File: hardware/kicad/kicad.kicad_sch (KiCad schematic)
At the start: 142 parts, among them J1 Conn_01x05, J2 USB_C_Receptacle_USB2.0, J3 Conn_01x08, SW1 MX_SW_solder, SW10 MX_SW_solder, SW11 MX_SW_solder, SW12 MX_SW_solder, SW13 MX_SW_solder, SW14 MX_SW_solder, SW15 MX_SW_solder, SW16 MX_SW_solder, SW17 MX_SW_solder, SW18 MX_SW_solder, SW19 MX_SW_solder, SW2 MX_SW_solder, SW20 MX_SW_solder, SW21 MX_SW_solder, SW22 MX_SW_solder, SW23 MX_SW_solder, SW24 MX_SW_solder, SW25 MX_SW_solder, SW26 MX_SW_solder, SW27 MX_SW_solder, SW28 MX_SW_solder, SW29 MX_SW_solder, SW3 MX_SW_solder, SW30 MX_SW_solder, SW31 MX_SW_solder, SW32 MX_SW_solder, SW33 MX_SW_solder, SW34 MX_SW_solder, SW35 MX_SW_solder, SW4 MX_SW_solder, SW5 MX_SW_solder, SW6 MX_SW_solder, SW7 MX_SW_solder, SW8 MX_SW_solder, SW9 MX_SW_solder, U1 RP2040, U2 W25Q128JVS, U3 XC6206PxxxMR, U4 USBLC6-2SC6, U5 74HC595, Y1 Crystal_GND24_Small

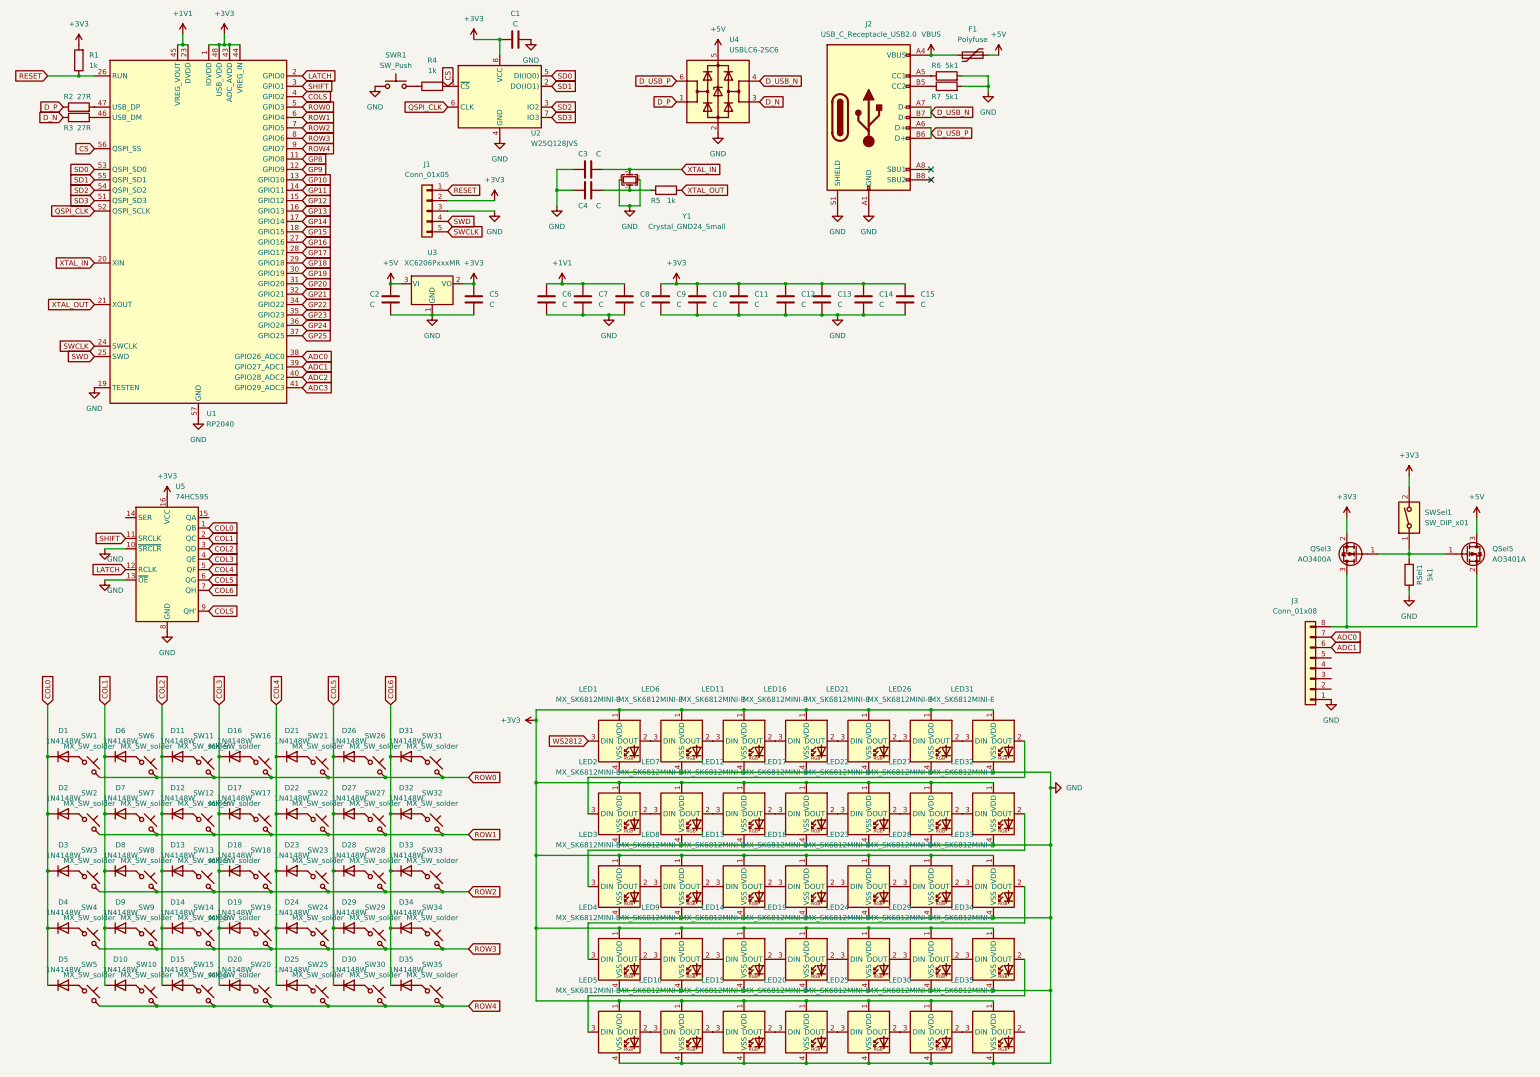
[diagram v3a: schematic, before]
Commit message: Update PCB
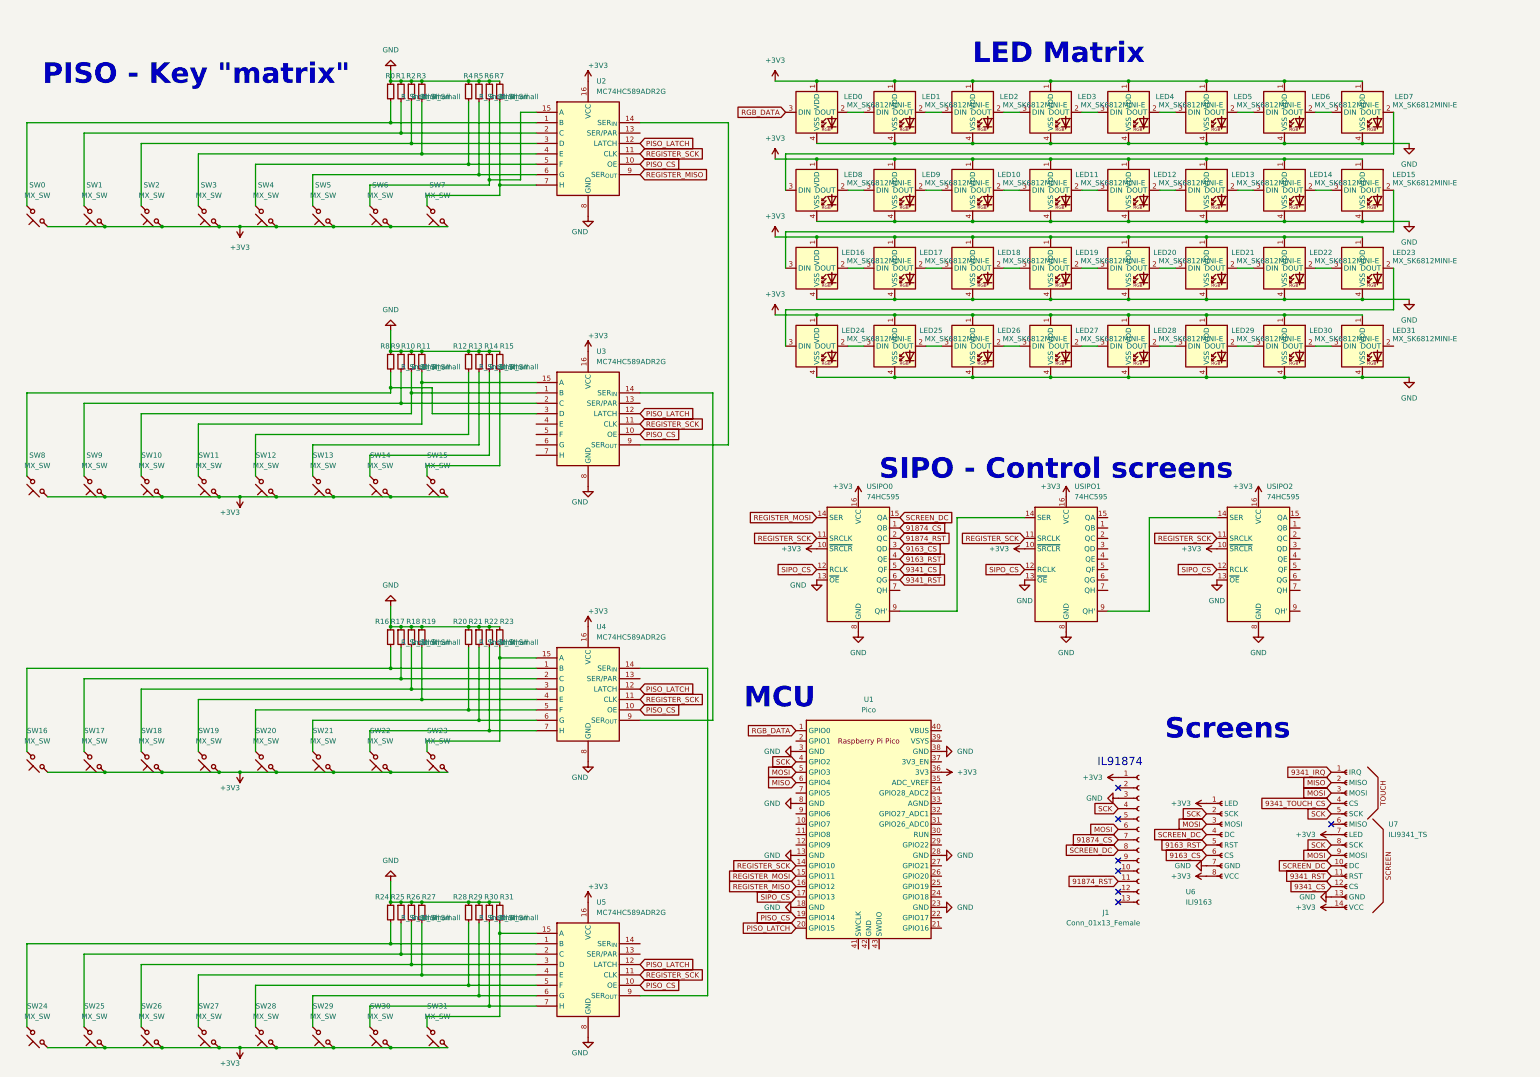
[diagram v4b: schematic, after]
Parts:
- removed C1, C10, C11, C12, C13, C14, C15, C2, C3, C4, C5, C6, C7, C8, C9: C, Capacitor_SMD:C_0603_1608Metric_Pad1.08x0.95mm_HandSolder, symbol Device:C
- removed D1, D10, D11, D12, D13, D14, D15, D16, D17, D18, D19, D2, D20, D21, D22, D23, D24, D25, D26, D27, D28, D29, D3, D30, D31, D32, D33, D34, D35, D4, D5, D6, D7, D8, D9: 1N4148W, Diode_SMD:D_SOD-123, symbol Diode:1N4148W
- removed F1: Polyfuse, Fuse:Fuse_0603_1608Metric_Pad1.05x0.95mm_HandSolder, symbol Device:Polyfuse
- removed J1: Conn_01x05, Connector_PinHeader_2.54mm:PinHeader_1x05_P2.54mm_Vertical, symbol Connector_Generic:Conn_01x05
- removed J2: USB_C_Receptacle_USB2.0, Connector_USB:USB_C_Receptacle_HRO_TYPE-C-31-M-12, symbol Connector:USB_C_Receptacle_USB2.0
- removed J3: Conn_01x08, Connector_PinHeader_2.54mm:PinHeader_1x08_P2.54mm_Vertical_SMD_Pin1Right, symbol Connector_Generic:Conn_01x08
- removed LED32, LED33, LED34, LED35: MX_SK6812MINI-E, marbastlib-mx:LED_MX_6028R, symbol marbastlib-mx:MX_SK6812MINI-E
- removed QSel3: AO3400A, Package_TO_SOT_SMD:SOT-23, symbol Transistor_FET:AO3400A
- removed QSel5: AO3401A, Package_TO_SOT_SMD:SOT-23, symbol Transistor_FET:AO3401A
- removed R1, R4, R5: 1k, Resistor_SMD:R_0603_1608Metric_Pad0.98x0.95mm_HandSolder, symbol Device:R
- removed R2, R3: 27R, Resistor_SMD:R_0603_1608Metric_Pad0.98x0.95mm_HandSolder, symbol Device:R
- removed R6, R7, RSel1: 5k1, Resistor_SMD:R_0603_1608Metric_Pad0.98x0.95mm_HandSolder, symbol Device:R
- removed SW1, SW10, SW11, SW12, SW13, SW14, SW15, SW16, SW17, SW18, SW19, SW2, SW20, SW21, SW22, SW23, SW24, SW25, SW26, SW27, SW28, SW29, SW3, SW30, SW31, SW32, SW33, SW34, SW35, SW4, SW5, SW6, SW7, SW8, SW9: MX_SW_solder, marbastlib-mx:SW_MX_1u, symbol marbastlib-mx:MX_SW_solder
- removed SWR1: SW_Push, Button_Switch_SMD:SW_SPST_TL3342, symbol Switch:SW_Push
- removed SWSel1: SW_DIP_x01, Button_Switch_SMD:SW_DIP_SPSTx01_Slide_6.7x4.1mm_W6.73mm_P2.54mm_LowProfile_JPin, symbol Switch:SW_DIP_x01
- removed U1: RP2040, Package_DFN_QFN:QFN-56-1EP_7x7mm_P0.4mm_EP3.2x3.2mm, symbol MCU_RaspberryPi:RP2040
- removed U2: W25Q128JVS, Package_SO:SOIC-8_5.23x5.23mm_P1.27mm, symbol Memory_Flash:W25Q128JVS
- removed U3: XC6206PxxxMR, Package_TO_SOT_SMD:SOT-23, symbol Regulator_Linear:XC6206PxxxMR
- removed U4: USBLC6-2SC6, Package_TO_SOT_SMD:SOT-23-6, symbol Power_Protection:USBLC6-2SC6
- removed U5: 74HC595, soic:SOIC16, symbol 74xx:74HC595
- removed Y1: Crystal_GND24_Small, Crystal:Crystal_SMD_3225-4Pin_3.2x2.5mm_HandSoldering, symbol Device:Crystal_GND24_Small
- added J1: Conn_01x13_Female, Connector_PinHeader_1.00mm:PinHeader_1x13_P1.00mm_Vertical, symbol Connector:Conn_01x13_Female
- added LED0: MX_SK6812MINI-E, marbastlib-mx:LED_MX_6028R, symbol marbastlib-mx:MX_SK6812MINI-E
- added R0, R1, R10, R11, R12, R13, R14, R15, R16, R17, R18, R19, R2, R20, R21, R22, R23, R24, R25, R26, R27, R28, R29, R3, R30, R31, R4, R5, R6, R7, R8, R9: R_Small, Resistor_SMD:R_1206_3216Metric_Pad1.30x1.75mm_HandSolder, symbol Device:R_Small
- added SW0, SW1, SW10, SW11, SW12, SW13, SW14, SW15, SW16, SW17, SW18, SW19, SW2, SW20, SW21, SW22, SW23, SW24, SW25, SW26, SW27, SW28, SW29, SW3, SW30, SW31, SW4, SW5, SW6, SW7, SW8, SW9: MX_SW, marbastlib-mx:SW_MX_1u, symbol marbastlib-mx:MX_SW_HS
- added U1: Pico, MCU_RaspberryPi_and_Boards:RPi_Pico_SMD_TH, symbol MCU_RaspberryPi_and_Boards:Pico
- added U2, U3, U4, U5: MC74HC589ADR2G, Package_SO:SO-16_3.9x9.9mm_P1.27mm, symbol my_components:MC74HC589ADR2G
- added U6: ILI9163, my_components:ILI9163, symbol my_components:ILI9163
- added U7: ILI9341_TS, my_components:ILI9341_TS, symbol my_components:ILI9341_TS
- added USIPO0, USIPO1, USIPO2: 74HC595, Package_SO:SO-16_3.9x9.9mm_P1.27mm, symbol 74xx:74HC595
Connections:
- net +3V3: now also J1.1 (Pin_1), LED0.1 (VDD), SW0.1, SW1.1, SW10.1, SW11.1, SW12.1, SW13.1, SW14.1, SW15.1, SW16.1, SW17.1, SW18.1, SW19.1, SW2.1, SW20.1, SW21.1, SW22.1, SW23.1, SW24.1, SW25.1, SW26.1, SW27.1, SW28.1, SW29.1, SW3.1, SW30.1, SW31.1, SW4.1, SW5.1, SW6.1, SW7.1, SW8.1, SW9.1, U1.36 (3V3), U2.16 (VCC), U3.16 (VCC), U4.16 (VCC), U5.16 (VCC), U6.1 (LED), U6.8 (VCC), U7.14 (VCC), U7.7 (LED), USIPO0.10 (~{SRCLR}), USIPO0.16 (VCC), USIPO1.10 (~{SRCLR}), USIPO1.16 (VCC), USIPO2.10 (~{SRCLR}), USIPO2.16 (VCC)
- net GND: now also J1.3 (Pin_3), LED0.4 (VSS), R0.1, R1.1, R10.1, R11.1, R12.1, R13.1, R14.1, R15.1, R16.1, R17.1, R18.1, R19.1, R2.1, R20.1, R21.1, R22.1, R23.1, R24.1, R25.1, R26.1, R27.1, R28.1, R29.1, R3.1, R30.1, R31.1, R4.1, R5.1, R6.1, R7.1, R8.1, R9.1, U1.13 (GND), U1.18 (GND), U1.23 (GND), U1.28 (GND), U1.3 (GND), U1.38 (GND), U1.8 (GND), U2.8 (GND), U3.8 (GND), U4.8 (GND), U5.8 (GND), U6.7 (GND), U7.13 (GND), USIPO0.13 (~{OE}), USIPO0.8 (GND), USIPO1.13 (~{OE}), USIPO1.8 (GND), USIPO2.13 (~{OE}), USIPO2.8 (GND)
- net at LED6.2 (DOUT): now also LED7.3 (DIN); no longer LED11.3 (DIN)
- net at LED1.2 (DOUT): now also LED2.3 (DIN); no longer LED6.3 (DIN)
- net at LED2.2 (DOUT): now also LED3.3 (DIN); no longer LED7.3 (DIN)
- net at LED31.2 (DOUT): no longer LED2.3 (DIN)
- net at LED22.3 (DIN): now also LED21.2 (DOUT); no longer LED17.2 (DOUT)
- net at LED12.2 (DOUT): now also LED13.3 (DIN); no longer LED17.3 (DIN)
- net at LED23.3 (DIN): now also LED22.2 (DOUT); no longer LED18.2 (DOUT)
- net at LED18.3 (DIN): now also LED17.2 (DOUT); no longer LED13.2 (DOUT)
- net at LED30.2 (DOUT): now also LED31.3 (DIN)
- net at LED28.3 (DIN): now also LED27.2 (DOUT); no longer LED23.2 (DOUT)
- net at LED29.2 (DOUT): now also LED30.3 (DIN)
- net at LED29.3 (DIN): now also LED28.2 (DOUT); no longer LED24.2 (DOUT)
- net at LED26.3 (DIN): now also LED25.2 (DOUT); no longer LED21.2 (DOUT)
- net at LED21.3 (DIN): now also LED20.2 (DOUT); no longer LED16.2 (DOUT)
- net at LED4.3 (DIN): now also LED3.2 (DOUT)
- net at LED26.2 (DOUT): now also LED27.3 (DIN); no longer LED31.3 (DIN)
- net at LED25.3 (DIN): now also LED24.2 (DOUT); no longer LED20.2 (DOUT)
- net at LED15.3 (DIN): now also LED14.2 (DOUT); no longer LED10.2 (DOUT)
- net at LED10.3 (DIN): now also LED9.2 (DOUT); no longer LED5.2 (DOUT)
- net at LED19.3 (DIN): now also LED18.2 (DOUT); no longer LED14.2 (DOUT)
- net at LED14.3 (DIN): now also LED13.2 (DOUT); no longer LED9.2 (DOUT)
- net at LED20.3 (DIN): now also LED19.2 (DOUT); no longer LED15.2 (DOUT)
- net at LED12.3 (DIN): now also LED11.2 (DOUT); no longer LED7.2 (DOUT)
- net at LED8.2 (DOUT): now also LED9.3 (DIN); no longer LED13.3 (DIN)
- net at LED8.3 (DIN): now also LED7.2 (DOUT); no longer LED3.2 (DOUT)
- net at LED24.3 (DIN): now also LED23.2 (DOUT); no longer LED19.2 (DOUT)
- net at LED4.2 (DOUT): now also LED5.3 (DIN); no longer LED9.3 (DIN)
- net at LED16.3 (DIN): now also LED15.2 (DOUT); no longer LED11.2 (DOUT)
- net WS2812: no longer names the net of LED1.3 (DIN)
- net WS2812: now also LED0.2 (DOUT)
- new net: R2.2, SW2.2, U2.3 (D)
- new net: R20.2, SW20.2, U4.5 (F)
- new net: R16.2, SW16.2, U4.1 (B)
- new net: R18.2, SW18.2, U4.3 (D)
- new net: R5.2, SW5.2, U2.6 (G)
- new net: R11.2, SW11.2, U3.15 (A)
- new net: R22.2, SW22.2, U4.7 (H)
- new net: R13.2, SW13.2
- new net: R9.2, SW9.2, U3.2 (C)
- new net: LED16.2 (DOUT), LED17.3 (DIN)
- new net: R31.2, SW31.2, U5.15 (A)
- new net: R6.2, SW6.2, U2.15 (A)
- new net: R3.2, SW3.2, U2.4 (E)
- new net: USIPO0.9 (QH'), USIPO1.14 (SER)
- new net: USIPO1.9 (QH'), USIPO2.14 (SER)
- new net: R14.2, SW14.2
- new net: R25.2, SW25.2, U5.2 (C)
- new net: R19.2, SW19.2, U4.4 (E)
- new net: R7.2, SW7.2, U2.7 (H)
- new net: R24.2, SW24.2, U5.1 (B)
- new net: R26.2, SW26.2, U5.3 (D)
- new net: R10.2, SW10.2, U3.1 (B)
- new net: U3.14 (SER_{IN}), U4.9 (SER_{OUT})
- new net: R8.2, SW8.2, U3.3 (D)
- new net: U2.14 (SER_{IN}), U3.9 (SER_{OUT})
- new net: U4.14 (SER_{IN}), U5.9 (SER_{OUT})
- new net: R23.2, SW23.2, U4.15 (A)
- new net: R17.2, SW17.2, U4.2 (C)
- new net: R21.2, SW21.2, U4.6 (G)
- new net: R4.2, SW4.2, U2.5 (F)
- new net: R1.2, SW1.2, U2.2 (C)
- new net: R30.2, SW30.2, U5.7 (H)
- new net: LED10.2 (DOUT), LED11.3 (DIN)
- new net: R12.2, SW12.2
- new net: R28.2, SW28.2, U5.5 (F)
- new net: R27.2, SW27.2, U5.4 (E)
- new net: R29.2, SW29.2, U5.6 (G)
- new net: R0.2, SW0.2, U2.1 (B)
- new net: R15.2, SW15.2
- new net: LED5.2 (DOUT), LED6.3 (DIN)
- new net 9163_CS: U6.6 (CS), USIPO0.3 (QD)
- new net 9163_RST: U6.5 (RST), USIPO0.4 (QE)
- new net 91874_CS: J1.7 (Pin_7), USIPO0.1 (QB)
- new net 91874_RST: J1.11 (Pin_11), USIPO0.2 (QC)
- new net 9341_CS: U7.12 (CS), USIPO0.5 (QF)
- new net 9341_IRQ: U7.1 (IRQ)
- new net 9341_RST: U7.11 (RST), USIPO0.6 (QG)
- new net 9341_TOUCH_CS: U7.4 (CS)
- new net MISO: U1.6 (GPIO4), U7.2 (MISO)
- new net MOSI: J1.6 (Pin_6), U1.5 (GPIO3), U6.3 (MOSI), U7.3 (MOSI), U7.9 (MOSI)
- new net PISO_CS: U1.19 (GPIO14), U2.10 (OE), U3.10 (OE), U4.10 (OE), U5.10 (OE)
- new net PISO_LATCH: U1.20 (GPIO15), U2.12 (LATCH), U3.12 (LATCH), U4.12 (LATCH), U5.12 (LATCH)
- new net REGISTER_MISO: U1.16 (GPIO12), U2.9 (SER_{OUT})
- new net REGISTER_MOSI: U1.15 (GPIO11), USIPO0.14 (SER)
- new net REGISTER_SCK: U1.14 (GPIO10), U2.11 (CLK), U3.11 (CLK), U4.11 (CLK), U5.11 (CLK), USIPO0.11 (SRCLK), USIPO1.11 (SRCLK), USIPO2.11 (SRCLK)
- new net RGB_DATA: LED0.3 (DIN), U1.1 (GPIO0)
- new net SCK: J1.4 (Pin_4), U1.4 (GPIO2), U6.2 (SCK), U7.5 (SCK), U7.8 (SCK)
- new net SCREEN_DC: J1.8 (Pin_8), U6.4 (DC), U7.10 (DC), USIPO0.15 (QA)
- new net SIPO_CS: U1.17 (GPIO13), USIPO0.12 (RCLK), USIPO1.12 (RCLK), USIPO2.12 (RCLK)
- no-connect marks 2 -> 7
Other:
- note added: "IL91874"
- note added: "LED Matrix"
- note added: "MCU"
- note added: "PISO - Key "matrix""
- note added: "SIPO - Control screens"
- note added: "Screens"
- title: (none) -> Access Keyboard

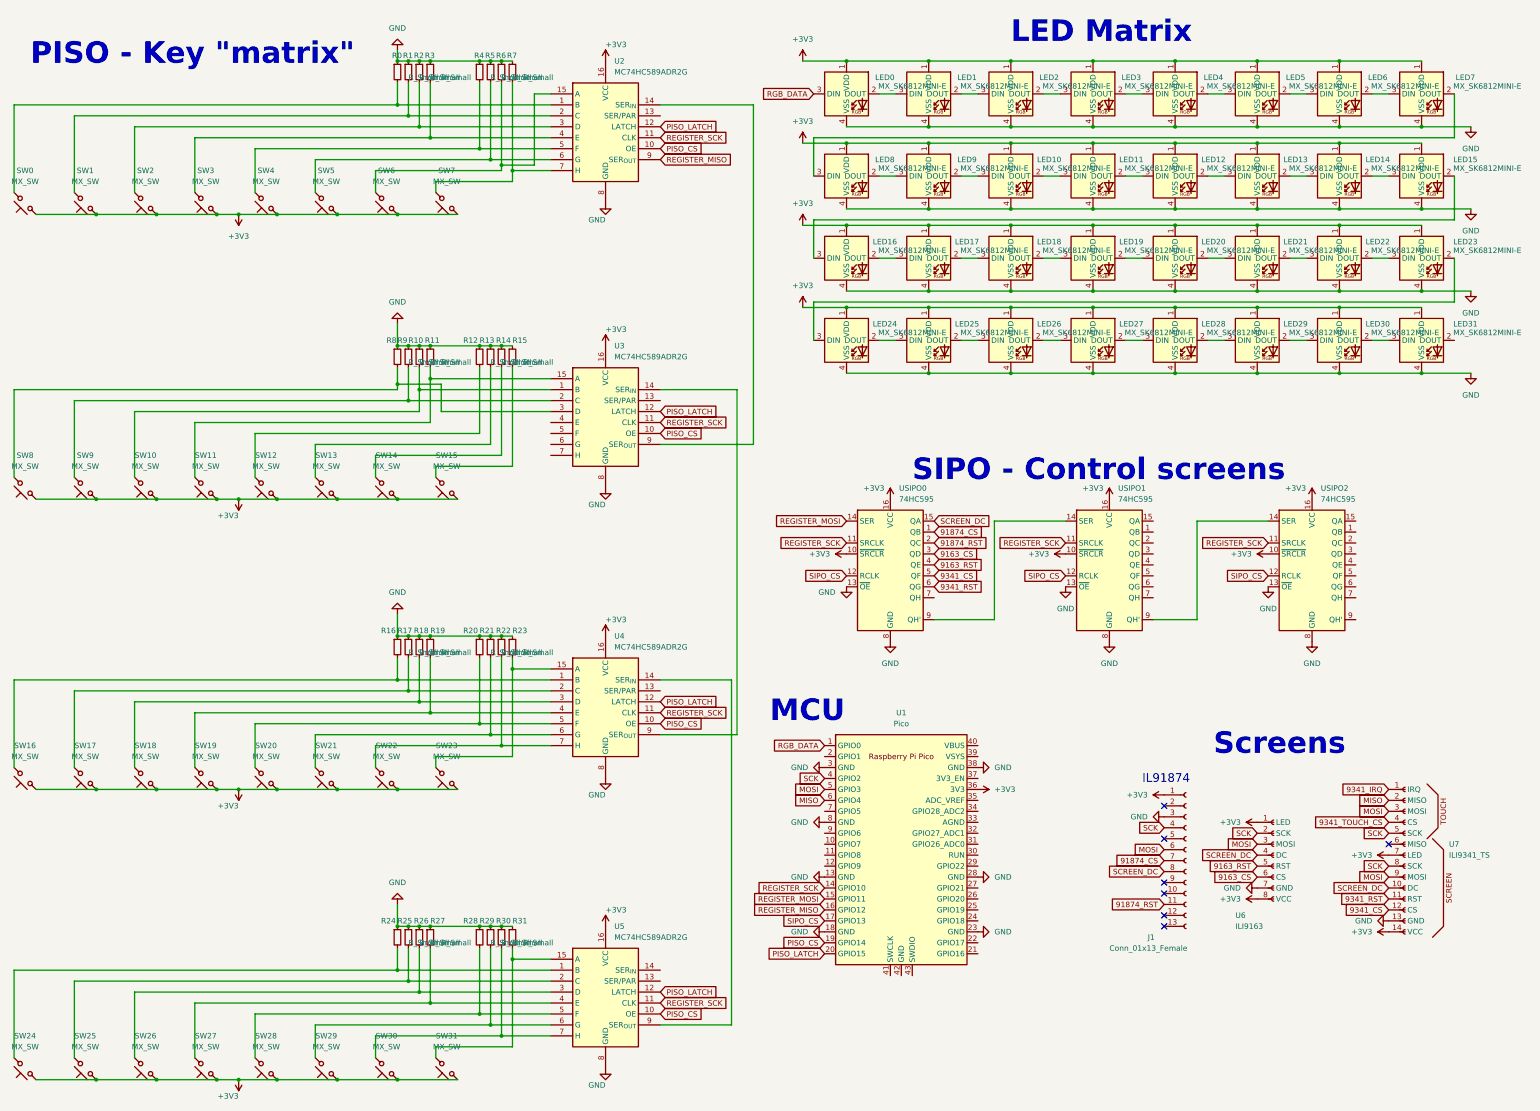
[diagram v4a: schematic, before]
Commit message: Matrix wired
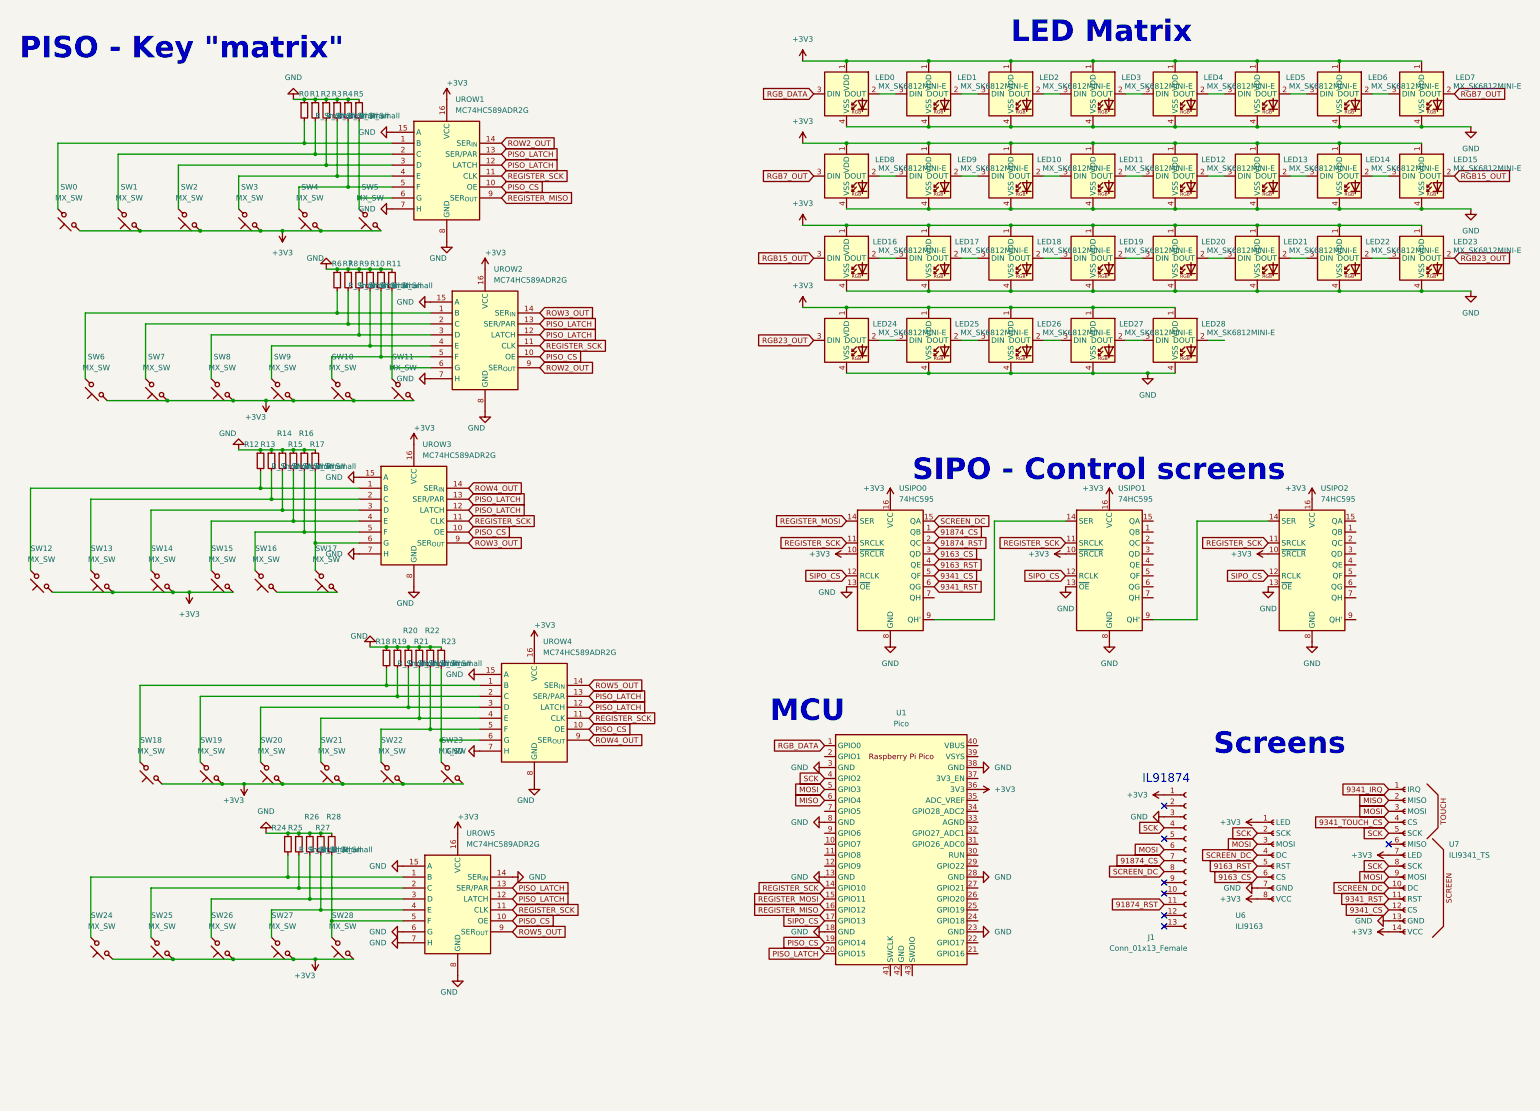
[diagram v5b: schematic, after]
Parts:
- removed LED29, LED30, LED31: MX_SK6812MINI-E, marbastlib-mx:LED_MX_6028R, symbol marbastlib-mx:MX_SK6812MINI-E
- removed R29, R30, R31: R_Small, Resistor_SMD:R_1206_3216Metric_Pad1.30x1.75mm_HandSolder, symbol Device:R_Small
- removed SW29, SW30, SW31: MX_SW, marbastlib-mx:SW_MX_1u, symbol marbastlib-mx:MX_SW_HS
- added UROW4: MC74HC589ADR2G, Package_SO:SO-16_3.9x9.9mm_P1.27mm, symbol my_components:MC74HC589ADR2G
- renumbered U2 to UROW1, U3 to UROW2, U4 to UROW3, U5 to UROW5
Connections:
- net +3V3: now also UROW4.16 (VCC); no longer SW16.1, SW17.1
- net GND: now also UROW1.15 (A), UROW1.7 (H), UROW2.15 (A), UROW2.7 (H), UROW3.15 (A), UROW3.7 (H), UROW5.14 (SER_{IN}), UROW5.15 (A), UROW5.6 (G), UROW5.7 (H), UROW4.15 (A), UROW4.7 (H), UROW4.8 (GND)
- net PISO_CS: now also UROW4.10 (OE)
- net PISO_LATCH: now also UROW1.13 (SER/PAR), UROW2.13 (SER/PAR), UROW3.13 (SER/PAR), UROW5.13 (SER/PAR), UROW4.12 (LATCH), UROW4.13 (SER/PAR)
- net REGISTER_SCK: now also UROW4.11 (CLK)
- net at R20.2, SW20.2: now also UROW4.3 (D); no longer UROW3.5 (F)
- net at R16.2, SW16.2: now also UROW3.5 (F); no longer UROW3.1 (B)
- net at R18.2, SW18.2: now also UROW4.1 (B); no longer UROW3.3 (D)
- net RGB7_OUT: now reaches LED7.2 (DOUT), LED8.3 (DIN)
- net at R11.2, SW11.2: now also UROW2.6 (G); no longer UROW2.15 (A)
- net at R22.2, SW22.2: now also UROW4.5 (F); no longer UROW3.7 (H)
- net at R13.2, SW13.2: now also UROW3.2 (C)
- net at R9.2, SW9.2: now also UROW2.4 (E); no longer UROW2.2 (C)
- net RGB15_OUT: now reaches LED15.2 (DOUT), LED16.3 (DIN)
- net at R6.2, SW6.2: now also UROW2.1 (B); no longer UROW1.15 (A)
- net at R14.2, SW14.2: now also UROW3.3 (D)
- net at R19.2, SW19.2: now also UROW4.2 (C); no longer UROW3.4 (E)
- net at R7.2, SW7.2: now also UROW2.2 (C); no longer UROW1.7 (H)
- net at R10.2, SW10.2: now also UROW2.5 (F); no longer UROW2.1 (B)
- net ROW3_OUT: now reaches UROW2.14 (SER_{IN}), UROW3.9 (SER_{OUT})
- net ROW2_OUT: now reaches UROW1.14 (SER_{IN}), UROW2.9 (SER_{OUT})
- net ROW4_OUT: now reaches UROW3.14 (SER_{IN})
- net ROW4_OUT: now also UROW4.9 (SER_{OUT}); no longer UROW5.9 (SER_{OUT})
- net at R23.2, SW23.2: now also UROW4.6 (G); no longer UROW3.15 (A)
- net at R17.2, SW17.2: now also UROW3.6 (G); no longer UROW3.2 (C)
- net at R21.2, SW21.2: now also UROW4.4 (E); no longer UROW3.6 (G)
- net RGB23_OUT: now reaches LED23.2 (DOUT), LED24.3 (DIN)
- net at R12.2, SW12.2: now also UROW3.1 (B)
- net at R15.2, SW15.2: now also UROW3.4 (E)
- new net: SW16.1, SW17.1
- new net ROW5_OUT: UROW4.14 (SER_{IN}), UROW5.9 (SER_{OUT})
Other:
- moved on the sheet: R0, R1, R10, R11, R12, R13, R14, R15, R16, R17, R18, R19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
